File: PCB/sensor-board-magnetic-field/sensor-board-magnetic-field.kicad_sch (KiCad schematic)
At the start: 8 parts, among them U2 MAGNETIC POGO CONN., U3 MAGNETIC POGO CONN.

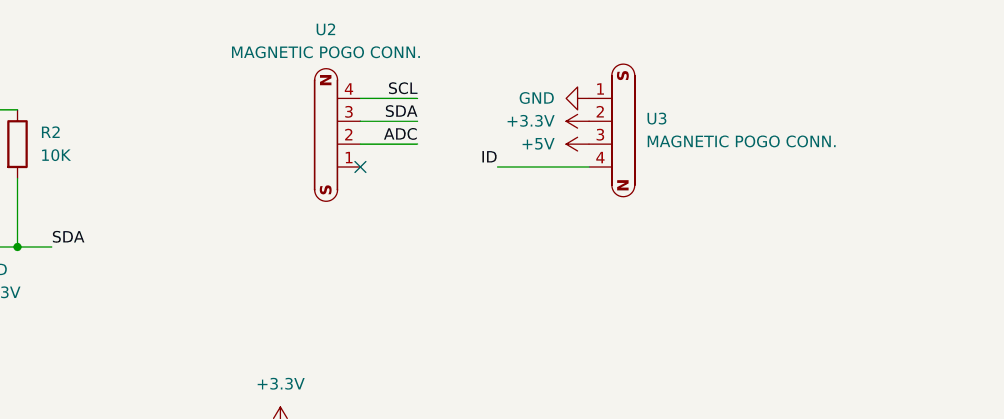
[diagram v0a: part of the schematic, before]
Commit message: made some changes
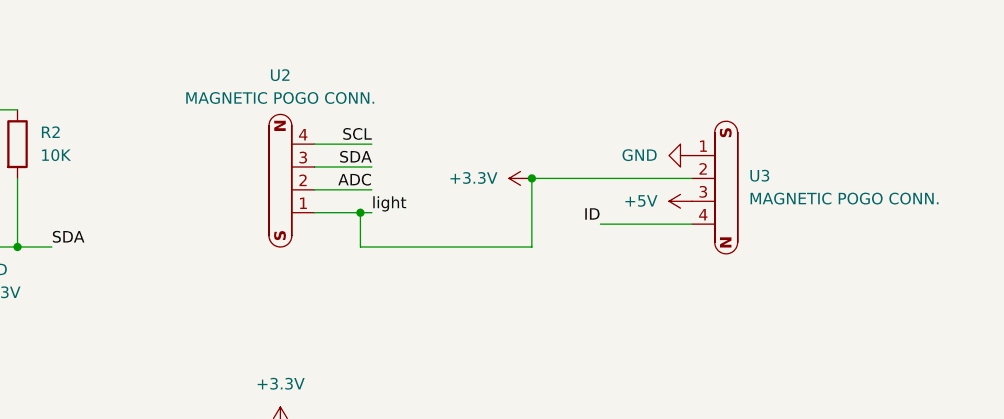
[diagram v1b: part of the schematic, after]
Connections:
- net +3.3V: now also U2.1
- no-connect marks 1 -> 0
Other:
- moved on the sheet: U3
